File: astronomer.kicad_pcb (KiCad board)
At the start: 2 copper layers, 150.7 x 99.3 mm, 83 parts, among them J1 6P6C, SW1 SW_Push_45deg, SW10 SW_Push_45deg, SW11 SW_Push_45deg, SW12 SW_Push_45deg, SW13 SW_Push_45deg, SW14 SW_Push_45deg, SW15 SW_Push_45deg, SW16 SW_Push_45deg, SW17 SW_Push_45deg, SW18 SW_Push_45deg, SW19 SW_Push_45deg, SW2 SW_Push_45deg, SW20 SW_Push_45deg, SW21 SW_Push_45deg, SW22 SW_Push_45deg, SW3 SW_Push_45deg, SW4 SW_Push_45deg, SW5 SW_Push_45deg, SW6 SW_Push_45deg, SW7 SW_Push_45deg, SW8 SW_Push_45deg, SW9 SW_Push_45deg, U2 SN74LV1T34DBV

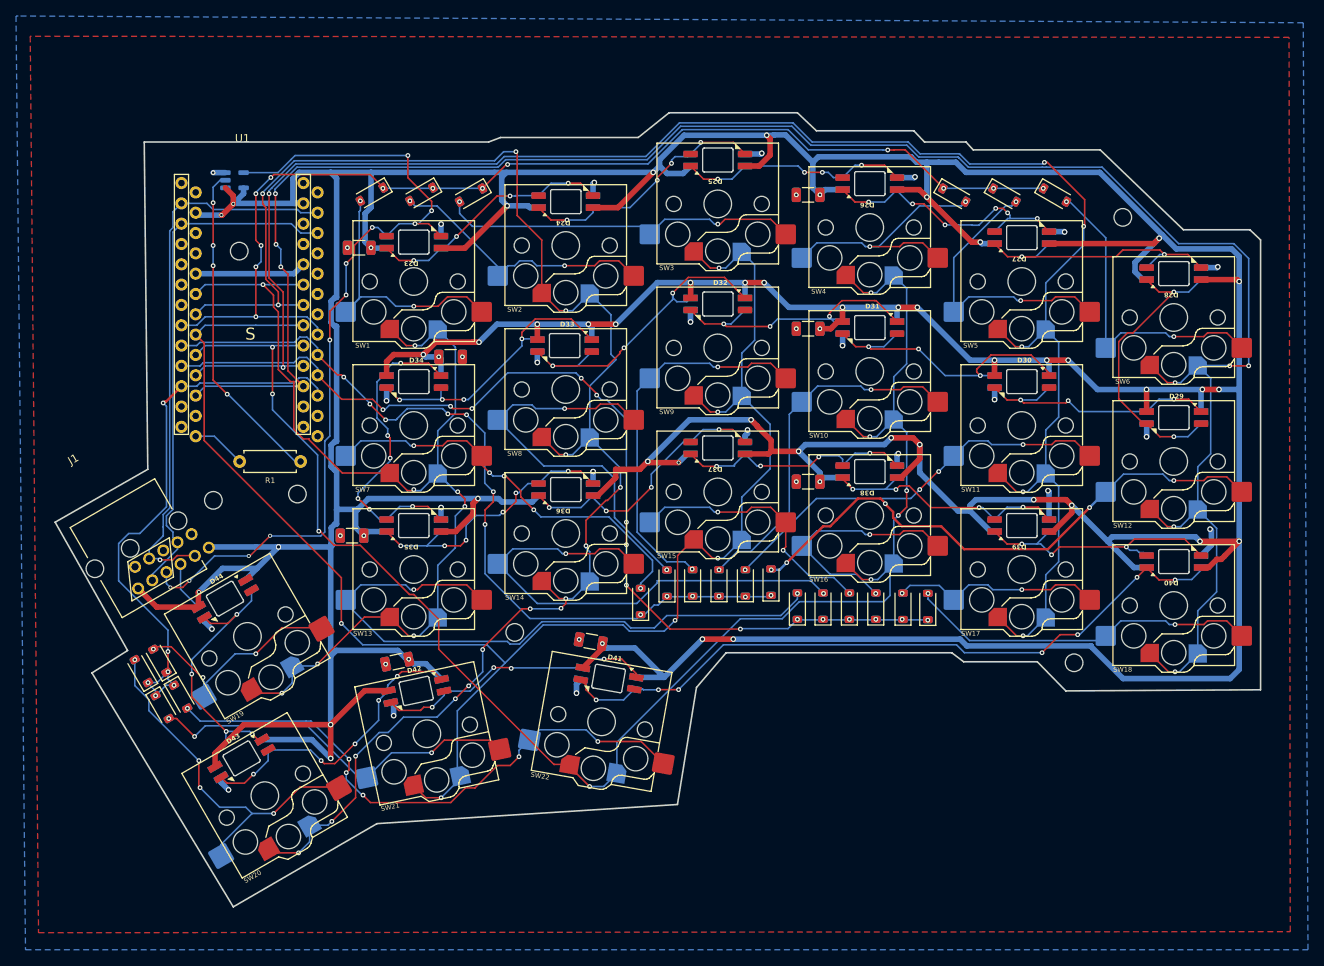
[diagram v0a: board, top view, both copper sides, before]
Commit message: Initial routing
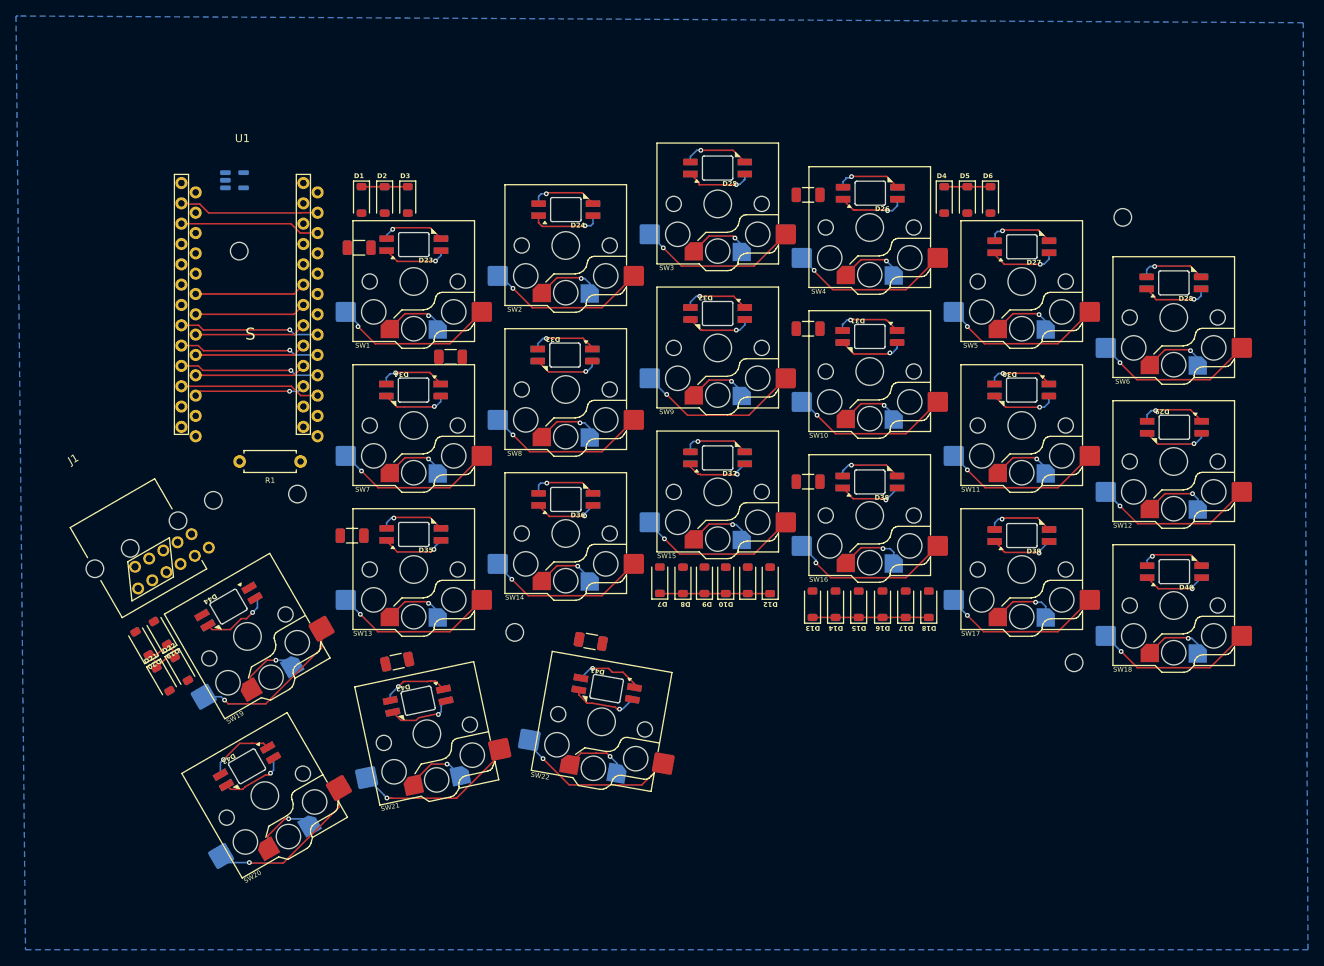
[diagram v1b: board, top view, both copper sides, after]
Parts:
- moved D6 7.88 mm to (238.2, 46.4), turned to -90 degrees
- moved D3 7.66 mm to (165.3, 46.4), turned to -90 degrees
- moved D5 4.52 mm to (235.3, 46.4), turned to -90 degrees
- moved D2 4.36 mm to (162.5, 46.4), turned to -90 degrees
- moved D7 3.59 mm to (195.9, 94.0)
- moved D20 3.47 mm to (131.2, 102.1)
- moved D21 3.47 mm to (134.7, 106.1)
- moved D19 3.47 mm to (133.5, 100.8)
- moved D22 3.47 mm to (137.0, 104.8)
- moved D8 2.02 mm to (198.7, 94.0)
- moved D13 1.91 mm to (214.9, 97.0)
- moved D14 1.59 mm to (217.8, 97.0)
- moved D9 1.52 mm to (201.4, 94.0)
- moved D4 1.44 mm to (232.4, 46.4), turned to -90 degrees
- moved D38 1.30 mm to (222.6, 81.7)
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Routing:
- net +5V: track 898.4 -> 0.00 mm, vias 51 -> 0
- net /Col 6: track 254.5 -> 38.8 mm, vias 8 -> 4
- net /Col 5: track 227.0 -> 38.6 mm, vias 7 -> 3
- net /Col 4: track 204.6 -> 46.7 mm, vias 9 -> 4
- net /Col 2: track 204.4 -> 46.5 mm, vias 16 -> 4
- net /Col 3: track 203.5 -> 46.1 mm, vias 6 -> 4
- net /Row 1: track 141.3 -> 29.1 mm, vias 13 -> 1
- net Net-(D23-DIN): track 107.5 -> 8.17 mm, vias 11 -> 1
- net /Row 3: track 125.5 -> 32.0 mm, vias 15 -> 1
- net /Col 1: track 137.4 -> 46.1 mm, vias 8 -> 4
- net Net-(D40-DOUT): track 88.2 -> 16.5 mm, vias 7 -> 2
- net /Row 2: track 103.0 -> 31.4 mm, vias 13 -> 1
- net Net-(D13-A): track 81.7 -> 20.3 mm, vias 2 -> 1
- net /TX: track 69.6 -> 17.5 mm, vias 1 -> 0
- net Net-(D22-A): track 72.4 -> 20.5 mm, vias 6 -> 1
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- added copper zone on B.Cu, net GND
- removed copper zone on B.Cu, net (none)
- removed copper zone on F.Cu, net GND
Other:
- board size 150.7 x 99.3 mm -> 4.6 x 4.4 mm
